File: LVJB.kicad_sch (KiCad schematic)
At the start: 18 parts, among them J1 Section H1, J10 Section F, J11 Section E1, J12 Section E2, J13 Section E3, J14 Section T1A, J2 Section A1, J3 Section A2, J4 Section A3, J5 Section A4, J6 Section M, J7 Section B1, J8 Section B2, J9 Section K

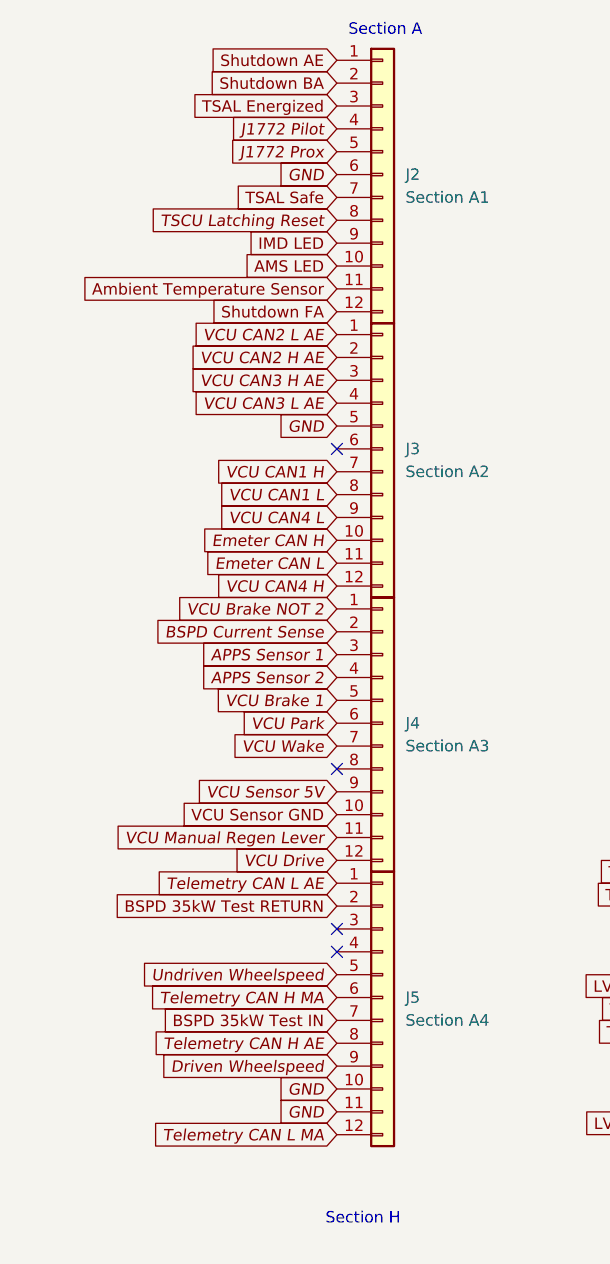
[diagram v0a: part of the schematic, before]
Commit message: 2mm wiring added
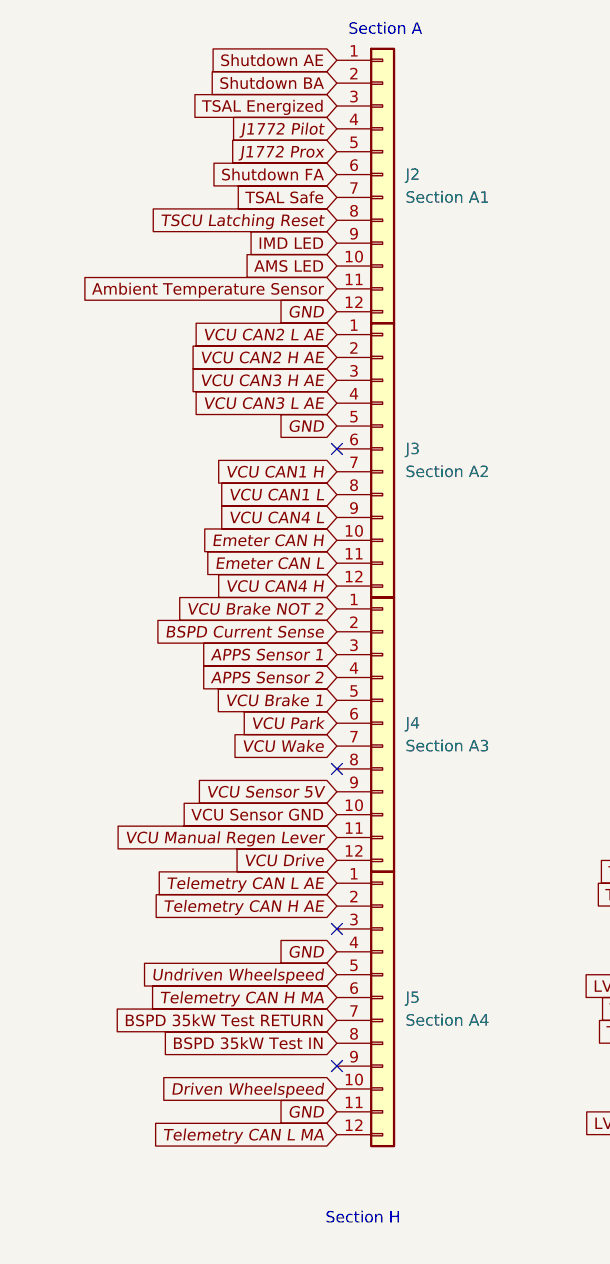
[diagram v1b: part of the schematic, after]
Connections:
- net BSPD 35kW Test IN: now also J5.8 (Pin_8); no longer J5.7 (Pin_7)
- net BSPD 35kW Test RETURN: now also J5.7 (Pin_7); no longer J5.2 (Pin_2)
- net Driven Wheelspeed: now also J5.10 (Pin_10); no longer J5.9 (Pin_9)
- net GND: now also J2.12 (Pin_12), J5.4 (Pin_4); no longer J2.6 (Pin_6), J5.10 (Pin_10)
- net Shutdown FA: now also J2.6 (Pin_6); no longer J2.12 (Pin_12)
- net Telemetry CAN H AE: now also J5.2 (Pin_2); no longer J5.8 (Pin_8)
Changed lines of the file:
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@@
   (paper "A4")
   (no_connect (at 227.33 64.77))
-  (no_connect (at 60.96 120.65))
+  (no_connect (at 60.96 133.35))
   (no_connect (at 60.96 118.11))
   (no_connect (at 189.23 95.25))
@@
     )
   )
-  (global_label "BSPD 35kW Test IN" (shape input) (at 60.96 128.27 180) (fields_autoplaced)
-    (effects (font (size 1.27 1.27)) (justify right))
-    (property "Intersheet References" "${INTERSHEET_REFS}" (id 0) (at 39.9807 128.1906 0)
-      (effects (font (size 1.27 1.27)) (justify right) hide)
-    )
-  )
   (global_label "VCU Brake NOT 2" (shape input) (at 241.3 140.97 0) (fields_autoplaced)
     (effects (font (size 1.27 1.27) italic) (justify left))
@@
     )
   )
+  (global_label "Driven Wheelspeed" (shape input) (at 60.96 135.89 180) (fields_autoplaced)
+    (effects (font (size 1.27 1.27) italic) (justify right))
+    (property "Intersheet References" "${INTERSHEET_REFS}" (id 0) (at 40.5113 135.8106 0)
+      (effects (font (size 1.27 1.27) italic) (justify right) hide)
+    )
+  )
   (global_label "IMD LED" (shape input) (at 60.96 41.91 180) (fields_autoplaced)
     (effects (font (size 1.27 1.27)) (justify right))
@@
     )
   )
+  (global_label "BSPD 35kW Test RETURN" (shape input) (at 60.96 128.27 180) (fields_autoplaced)
+    (effects (font (size 1.27 1.27)) (justify right))
+    (property "Intersheet References" "${INTERSHEET_REFS}" (id 0) (at 34.5983 128.1906 0)
+      (effects (font (size 1.27 1.27)) (justify right) hide)
+    )
+  )
   (global_label "VCU CAN1 H" (shape input) (at 60.96 67.31 180) (fields_autoplaced)
     (effects (font (size 1.27 1.27) italic) (justify right))
@@
     (effects (font (size 1.27 1.27) italic) (justify right))
     (property "Intersheet References" "${INTERSHEET_REFS}" (id 0) (at 41.5394 82.4706 0)
+      (effects (font (size 1.27 1.27) italic) (justify right) hide)
+    )
+  )
+  (global_label "GND" (shape input) (at 60.96 49.53 180) (fields_autoplaced)
+    (effects (font (size 1.27 1.27) italic) (justify right))
+    (property "Intersheet References" "${INTERSHEET_REFS}" (id 0) (at 54.4208 49.4506 0)
       (effects (font (size 1.27 1.27) italic) (justify right) hide)
     )
@@
     )
   )
-  (global_label "Shutdown FA" (shape input) (at 60.96 49.53 180) (fields_autoplaced)
-    (effects (font (size 1.27 1.27)) (justify right))
-    (property "Intersheet References" "${INTERSHEET_REFS}" (id 0) (at 46.3912 49.4506 0)
-      (effects (font (size 1.27 1.27)) (justify right) hide)
-    )
-  )
   (global_label "Telemetry CAN H AE" (shape input) (at 189.23 151.13 180) (fields_autoplaced)
     (effects (font (size 1.27 1.27)) (justify right))
@@
     )
   )
-  (global_label "Telemetry CAN H AE" (shape input) (at 60.96 130.81 180) (fields_autoplaced)
-    (effects (font (size 1.27 1.27) italic) (justify right))
-    (property "Intersheet References" "${INTERSHEET_REFS}" (id 0) (at 39.0599 130.7306 0)
-      (effects (font (size 1.27 1.27) italic) (justify right) hide)
-    )
-  )
   (global_label "VCU CAN2 H HB" (shape input) (at 59.69 170.18 180) (fields_autoplaced)
     (effects (font (size 1.27 1.27) italic) (justify right))
@@
     )
   )
+  (global_label "Telemetry CAN H AE" (shape input) (at 60.96 115.57 180) (fields_autoplaced)
+    (effects (font (size 1.27 1.27) italic) (justify right))
+    (property "Intersheet References" "${INTERSHEET_REFS}" (id 0) (at 39.0599 115.4906 0)
+      (effects (font (size 1.27 1.27) italic) (justify right) hide)
+    )
+  )
   (global_label "AMS LED" (shape input) (at 128.27 76.2 180) (fields_autoplaced)
     (effects (font (size 1.27 1.27) italic) (justify right))
@@
     )
   )
+  (global_label "BSPD 35kW Test IN" (shape input) (at 60.96 130.81 180) (fields_autoplaced)
+    (effects (font (size 1.27 1.27)) (justify right))
+    (property "Intersheet References" "${INTERSHEET_REFS}" (id 0) (at 39.9807 130.7306 0)
+      (effects (font (size 1.27 1.27)) (justify right) hide)
+    )
+  )
   (global_label "TSAL Energized" (shape input) (at 60.96 26.67 180) (fields_autoplaced)
     (effects (font (size 1.27 1.27)) (justify right))
@@
     (effects (font (size 1.27 1.27) italic) (justify right))
     (property "Intersheet References" "${INTERSHEET_REFS}" (id 0) (at 48.9175 110.4106 0)
+      (effects (font (size 1.27 1.27) italic) (justify right) hide)
+    )
+  )
+  (global_label "GND" (shape input) (at 60.96 120.65 180) (fields_autoplaced)
+    (effects (font (size 1.27 1.27) italic) (justify right))
+    (property "Intersheet References" "${INTERSHEET_REFS}" (id 0) (at 54.4208 120.5706 0)
       (effects (font (size 1.27 1.27) italic) (justify right) hide)
     )
@@
     )
   )
+  (global_label "Shutdown FA" (shape input) (at 60.96 34.29 180) (fields_autoplaced)
+    (effects (font (size 1.27 1.27)) (justify right))
+    (property "Intersheet References" "${INTERSHEET_REFS}" (id 0) (at 46.3912 34.2106 0)
+      (effects (font (size 1.27 1.27)) (justify right) hide)
+    )
+  )
   (global_label "VCU Brake 1" (shape input) (at 128.27 43.18 180) (fields_autoplaced)
     (effects (font (size 1.27 1.27) italic) (justify right))
@@
     )
   )
-  (global_label "GND" (shape input) (at 60.96 135.89 180) (fields_autoplaced)
-    (effects (font (size 1.27 1.27) italic) (justify right))
-    (property "Intersheet References" "${INTERSHEET_REFS}" (id 0) (at 54.4208 135.8106 0)
-      (effects (font (size 1.27 1.27) italic) (justify right) hide)
-    )
-  )
-  (global_label "GND" (shape input) (at 60.96 34.29 180) (fields_autoplaced)
-    (effects (font (size 1.27 1.27) italic) (justify right))
-    (property "Intersheet References" "${INTERSHEET_REFS}" (id 0) (at 54.4208 34.2106 0)
-      (effects (font (size 1.27 1.27) italic) (justify right) hide)
-    )
-  )
   (global_label "Shutdown AE" (shape input) (at 189.23 85.09 180) (fields_autoplaced)
     (effects (font (size 1.27 1.27)) (justify right))
@@
     )
   )
-  (global_label "Driven Wheelspeed" (shape input) (at 60.96 133.35 180) (fields_autoplaced)
-    (effects (font (size 1.27 1.27) italic) (justify right))
-    (property "Intersheet References" "${INTERSHEET_REFS}" (id 0) (at 40.5113 133.2706 0)
-      (effects (font (size 1.27 1.27) italic) (justify right) hide)
-    )
-  )
   (global_label "GND" (shape input) (at 133.35 176.53 180) (fields_autoplaced)
     (effects (font (size 1.27 1.27) italic) (justify right))
@@
     )
   )
-  (global_label "BSPD 35kW Test RETURN" (shape input) (at 60.96 115.57 180) (fields_autoplaced)
-    (effects (font (size 1.27 1.27)) (justify right))
-    (property "Intersheet References" "${INTERSHEET_REFS}" (id 0) (at 34.5983 115.4906 0)
-      (effects (font (size 1.27 1.27)) (justify right) hide)
-    )
-  )

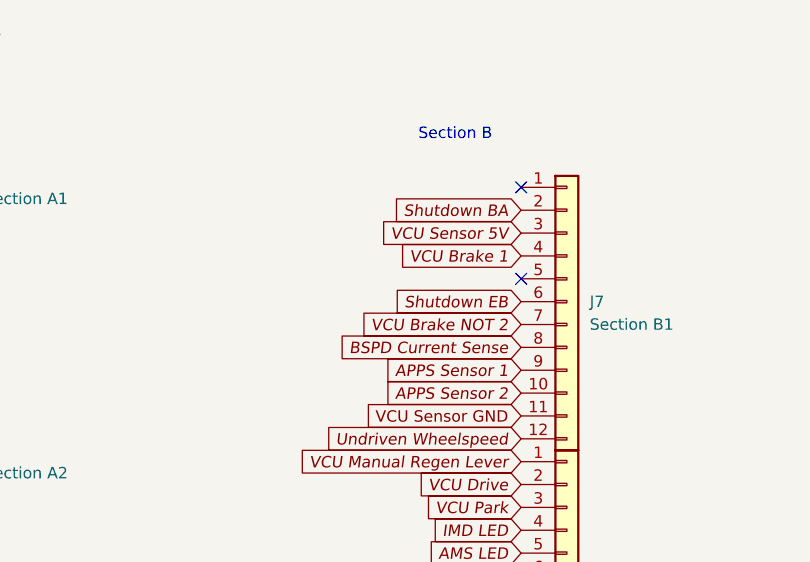
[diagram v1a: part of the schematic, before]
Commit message: Harness B extra conn added
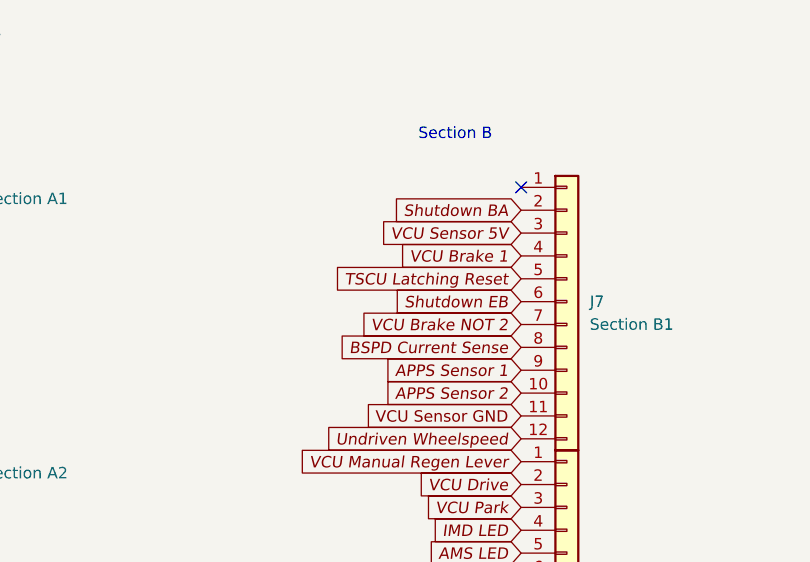
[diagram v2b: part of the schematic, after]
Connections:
- net TSCU Latching Reset: now also J7.5 (Pin_5)
- no-connect marks 22 -> 21
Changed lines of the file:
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@@
   (no_connect (at 189.23 92.71))
   (no_connect (at 189.23 90.17))
-  (no_connect (at 128.27 45.72))
   (no_connect (at 128.27 35.56))
   (no_connect (at 60.96 100.33))
@@
       (effects (font (size 1.27 1.27) italic) (justify right) hide)
     )
+  )
+  (global_label "TSCU Latching Reset" (shape input) (at 128.27 45.72 180) (fields_autoplaced)
+    (effects (font (size 1.27 1.27) italic) (justify right))
+    (property "Intersheet References" "${INTERSHEET_REFS}" (id 0) (at 105.6442 45.6406 0)
+      (effects (font (size 1.27 1.27) italic) (justify right) hide)
+    )

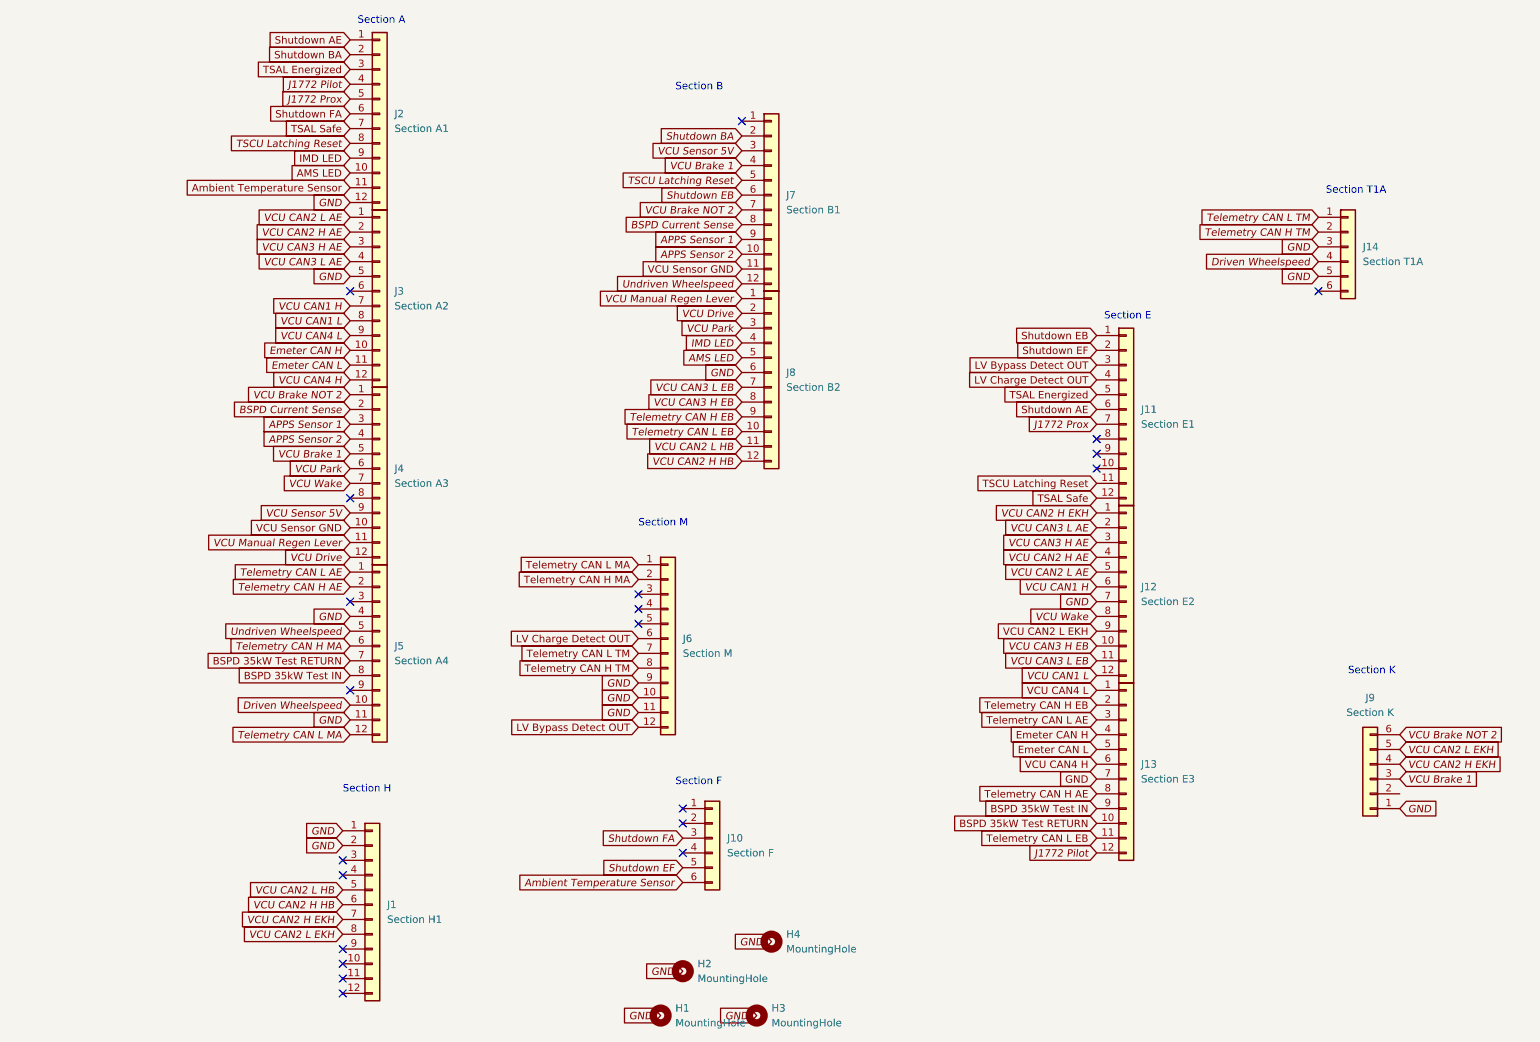
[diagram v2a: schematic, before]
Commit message: Fixed harness A
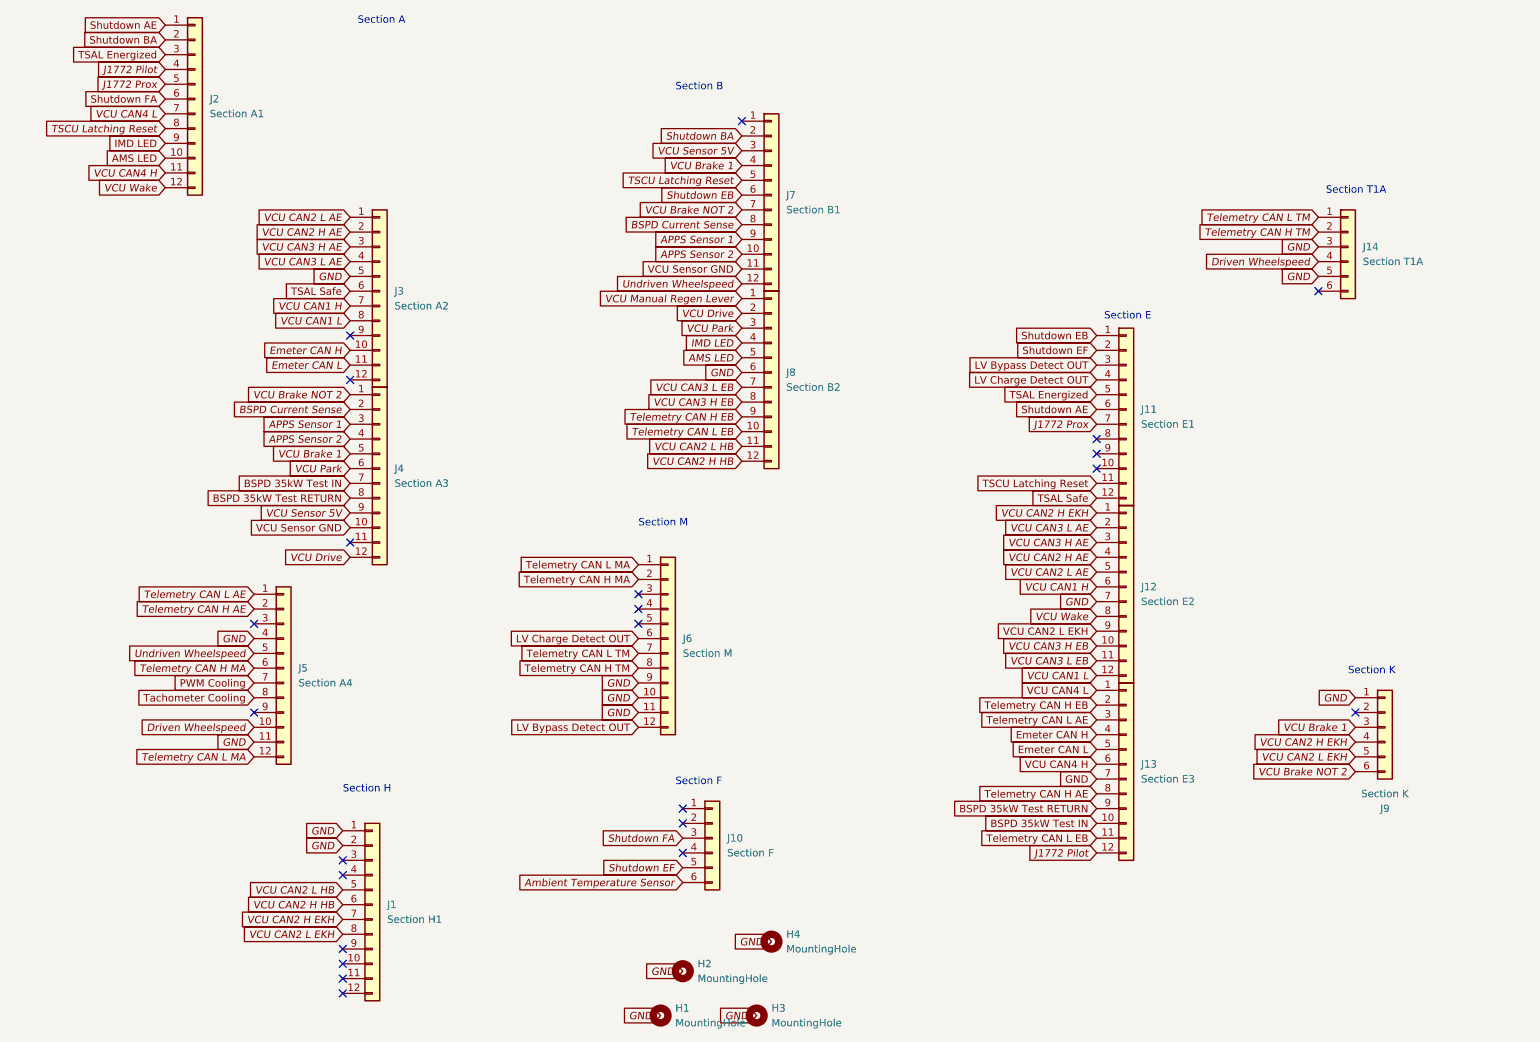
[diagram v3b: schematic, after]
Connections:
- net Ambient Temperature Sensor: no longer J2.11 (Pin_11)
- net BSPD 35kW Test IN: now also J13.10 (Pin_10), J4.7 (Pin_7); no longer J13.9 (Pin_9), J5.8 (Pin_8)
- net BSPD 35kW Test RETURN: now also J13.9 (Pin_9), J4.8 (Pin_8); no longer J13.10 (Pin_10), J5.7 (Pin_7)
- net GND: no longer J2.12 (Pin_12)
- net TSAL Safe: now also J3.6 (Pin_6); no longer J2.7 (Pin_7)
- net VCU CAN4 H: now also J2.11 (Pin_11); no longer J3.12 (Pin_12)
- net VCU CAN4 L: now also J2.7 (Pin_7); no longer J3.9 (Pin_9)
- net VCU Manual Regen Lever: no longer J4.11 (Pin_11)
- net VCU Wake: now also J2.12 (Pin_12); no longer J4.7 (Pin_7)
- new net PWM Cooling: J5.7 (Pin_7)
- new net Tachometer Cooling: J5.8 (Pin_8)
- no-connect marks 21 -> 23
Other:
- moved on the sheet: J2, J5, J9
